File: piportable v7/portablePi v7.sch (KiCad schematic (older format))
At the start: 62 parts, among them IC1 Raspberry_Pi_Zero_W_(v1.3), J1 AudioJack3, SW0 SW_Push, SW1 SW_Push, SW10 SW_Push, SW11 SW_Push, SW12 SW_Push, SW13 SW_Push, SW14 SW_Push, SW15 SW_Push, SW16 SW_Push, SW17 SW_Push, SW18 SW_Push, SW19 SW_Push, SW2 SW_Push, SW20 SW_Push, SW21 SW_Push, SW22 SW_Push, SW23 SW_Push, SW24 SW_Push, SW25 SW_Push, SW26 SW_Push, SW27 SW_Push, SW28 SW_Push, SW29 SW_Push, SW3 SW_Push, SW30 SW_Push, SW31 SW_Push, SW32 SW_Push, SW33 SW_Push, SW34 SW_Push, SW35 SW_Push, SW36 SW_Push, SW37 SW_Push, SW38 SW_Push, SW39 SW_Push, SW4 SW_Push, SW40 SW_Push, SW41 SW_Push, SW42 SW_Push, SW43 SW_Push, SW44 SW_Push, SW45 SW_Push, SW46 SW_Push, SW47 SW_Push, SW48 SW_Push, SW49 SW_Push, SW5 SW_Push, SW50 SW_Push, SW51 SW_Push, SW52 SW_Push, SW53 SW_Push, SW54 SW_Push, SW55 SW_Push, SW56 SW_Push, SW6 SW_Push, SW7 SW_Push, SW8 SW_Push, SW9 SW_Push, U1 ATmega328P-PU

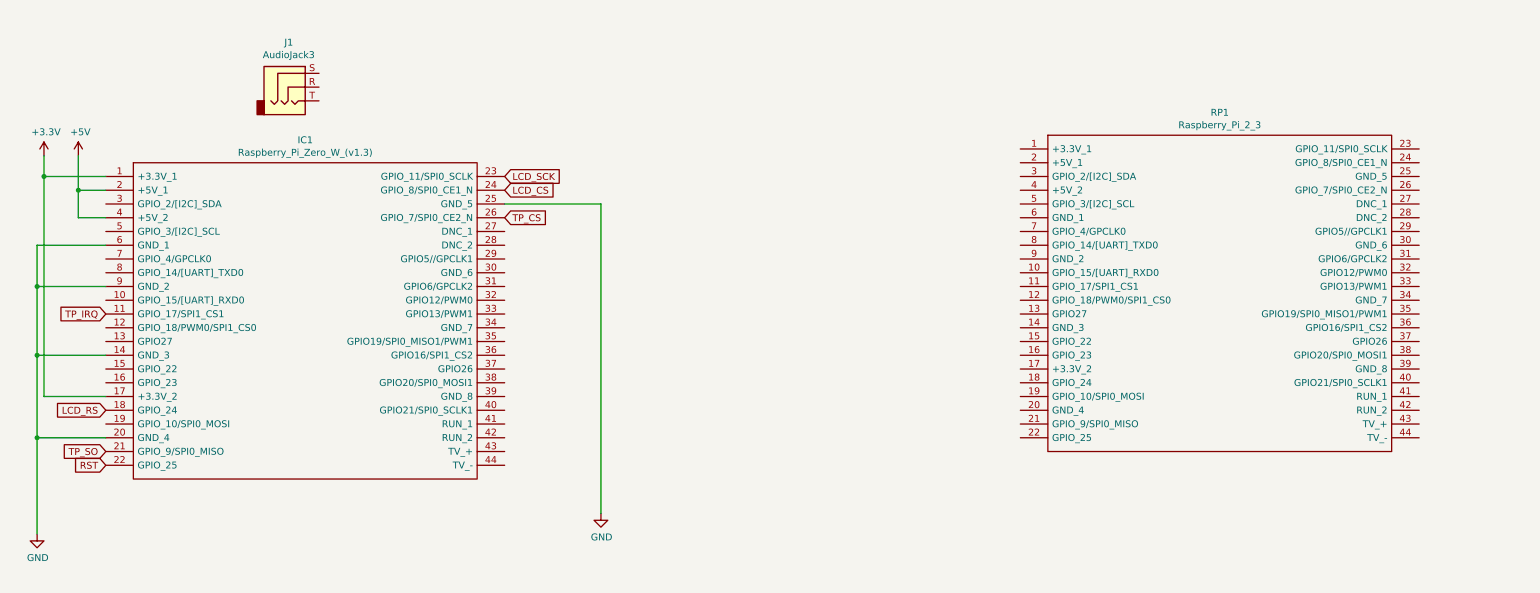
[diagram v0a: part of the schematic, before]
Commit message: nothing new
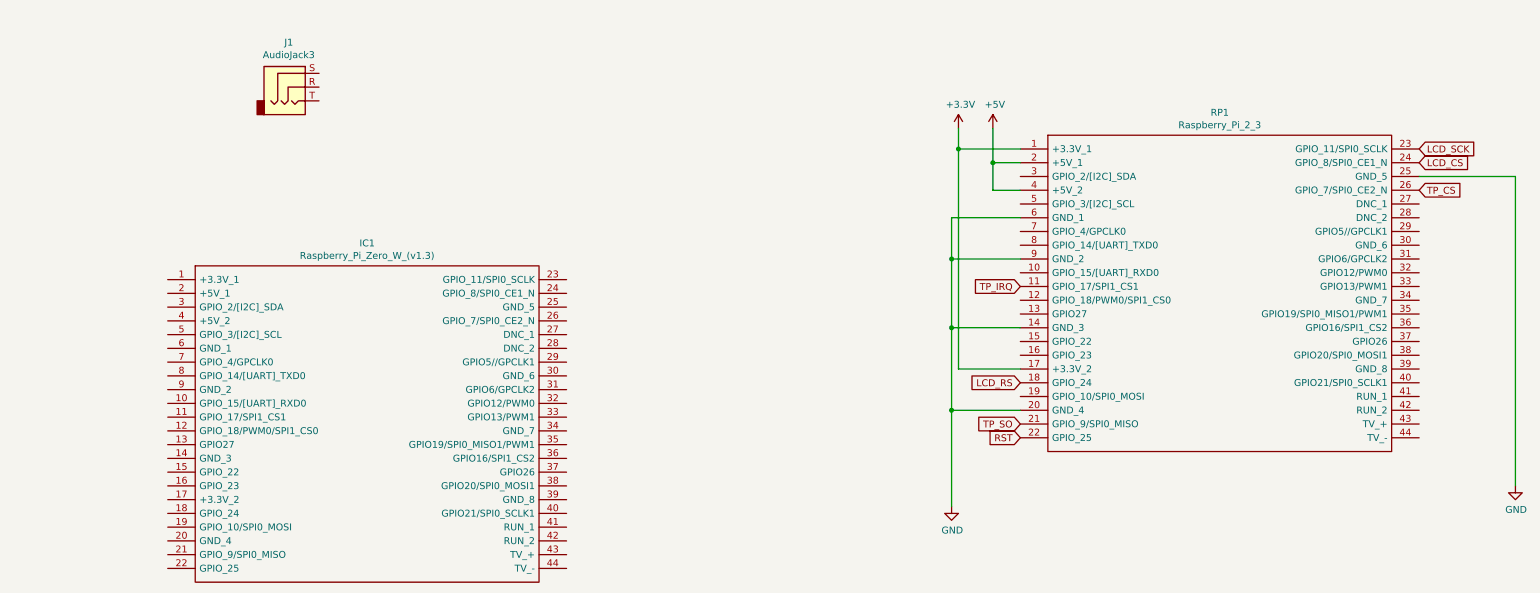
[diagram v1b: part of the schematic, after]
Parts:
- DS1: footprint pi2:raspberrypi_2_3 -> 35 display:3.5 inch RPi LCD
- RP1: footprint RASPBERRYPI -> (none)
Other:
- moved on the sheet: IC1
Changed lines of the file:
@@
 F 0 "DS1" H 2550 6647 50  0000 C CNN
 F 1 "3.5_Inch_RPI" H 2550 6556 50  0000 C CNN
-F 2 "pi2:raspberrypi_2_3" H 2550 5300 50  0001 C CNN
+F 2 "35 display:3.5 inch RPi LCD" H 2550 5300 50  0001 C CNN
 F 3 "DOCUMENTATION" H 2550 5300 50  0001 C CNN
 F 4 "https://www.elecrow.com/35-inch-480x320-tft-display-with-touch-screen-for-raspberry-pi-p-1385.html" H 2550 6465 50  0000 C CNN "Link"
@@
 L Raspberry_Pi_Zero_W_(v1.3):Raspberry_Pi_Zero_W_(v1.3) IC1
 U 1 1 5C56055C
-P 1350 7650
-F 0 "IC1" H 2800 7915 50  0000 C CNN
-F 1 "Raspberry_Pi_Zero_W_(v1.3)" H 2800 7824 50  0000 C CNN
-F 2 "pi2:raspberrypi_2_3" H 4100 7750 50  0001 L CNN
-F 3 "https://cdn.sparkfun.com/assets/learn_tutorials/6/7/6/PiZero_1.pdf" H 4100 7650 50  0001 L CNN
-F 4 "Raspberry Pi Zero W (v1.3) Single-board Computers" H 4100 7550 50  0001 L CNN "Description"
-F 5 "" H 4100 7450 50  0001 L CNN "Height"
-F 6 "RASPBERRY-PI" H 4100 7350 50  0001 L CNN "Manufacturer_Name"
-F 7 "Raspberry Pi Zero W (v1.3)" H 4100 7250 50  0001 L CNN "Manufacturer_Part_Number"
-F 8 "" H 4100 7150 50  0001 L CNN "RS Part Number"
-F 9 "" H 4100 7050 50  0001 L CNN "RS Price/Stock"
-F 10 "" H 4100 6950 50  0001 L CNN "Mouser Part Number"
-F 11 "" H 4100 6850 50  0001 L CNN "Mouser Price/Stock"
-	1    1350 7650
+P 1800 8400
+F 0 "IC1" H 3250 8665 50  0000 C CNN
+F 1 "Raspberry_Pi_Zero_W_(v1.3)" H 3250 8574 50  0000 C CNN
+F 2 "pi2:raspberrypi_2_3" H 4550 8500 50  0001 L CNN
+F 3 "https://cdn.sparkfun.com/assets/learn_tutorials/6/7/6/PiZero_1.pdf" H 4550 8400 50  0001 L CNN
+F 4 "Raspberry Pi Zero W (v1.3) Single-board Computers" H 4550 8300 50  0001 L CNN "Description"
+F 5 "" H 4550 8200 50  0001 L CNN "Height"
+F 6 "RASPBERRY-PI" H 4550 8100 50  0001 L CNN "Manufacturer_Name"
+F 7 "Raspberry Pi Zero W (v1.3)" H 4550 8000 50  0001 L CNN "Manufacturer_Part_Number"
+F 8 "" H 4550 7900 50  0001 L CNN "RS Part Number"
+F 9 "" H 4550 7800 50  0001 L CNN "RS Price/Stock"
+F 10 "" H 4550 7700 50  0001 L CNN "Mouser Part Number"
+F 11 "" H 4550 7600 50  0001 L CNN "Mouser Price/Stock"
+	1    1800 8400
 	1    0    0    -1
 $EndComp
@@
 Wire Wire Line
 	750  5800 750  6150
-Text GLabel 1350 9350 0    50   Input ~ 0
-LCD_RS
-Text GLabel 1350 9750 0    50   Input ~ 0
-RST
-Text GLabel 4250 7750 2    50   Input ~ 0
-LCD_CS
-Text GLabel 4250 7950 2    50   Input ~ 0
-TP_CS
-Text GLabel 1350 9650 0    50   Input ~ 0
-TP_SO
-Text GLabel 4250 7650 2    50   Input ~ 0
-LCD_SCK
-Text GLabel 1350 8650 0    50   Input ~ 0
-TP_IRQ
-$Comp
-L power:GND #PWR0105
-U 1 1 5C63ADD4
-P 4950 10100
-F 0 "#PWR0105" H 4950 9850 50  0001 C CNN
-F 1 "GND" H 4955 9927 50  0000 C CNN
-F 2 "" H 4950 10100 50  0001 C CNN
-F 3 "" H 4950 10100 50  0001 C CNN
-	1    4950 10100
-	1    0    0    -1
-$EndComp
-Wire Wire Line
-	4250 7850 4950 7850
-Wire Wire Line
-	4950 7850 4950 10100
-$Comp
-L power:GND #PWR0106
-U 1 1 5C641F49
-P 850 10250
-F 0 "#PWR0106" H 850 10000 50  0001 C CNN
-F 1 "GND" H 855 10077 50  0000 C CNN
-F 2 "" H 850 10250 50  0001 C CNN
-F 3 "" H 850 10250 50  0001 C CNN
-	1    850  10250
-	1    0    0    -1
-$EndComp
-Wire Wire Line
-	1350 9550 850  9550
-Wire Wire Line
-	850  9550 850  10250
-Wire Wire Line
-	1350 8950 850  8950
-Wire Wire Line
-	850  8950 850  9550
-Connection ~ 850  9550
-Wire Wire Line
-	1350 8450 850  8450
-Wire Wire Line
-	850  8450 850  8950
-Connection ~ 850  8950
-Wire Wire Line
-	1350 8150 850  8150
-Wire Wire Line
-	850  8150 850  8450
-Connection ~ 850  8450
-$Comp
-L power:+5V #PWR0107
-U 1 1 5C66060B
-P 1150 7500
-F 0 "#PWR0107" H 1150 7350 50  0001 C CNN
-F 1 "+5V" H 1165 7673 50  0000 C CNN
-F 2 "" H 1150 7500 50  0001 C CNN
-F 3 "" H 1150 7500 50  0001 C CNN
-	1    1150 7500
-	1    0    0    -1
-$EndComp
-Wire Wire Line
-	1150 7500 1150 7750
-Wire Wire Line
-	1150 7750 1350 7750
-Wire Wire Line
-	1350 7950 1150 7950
-Wire Wire Line
-	1150 7950 1150 7750
-Connection ~ 1150 7750
-$Comp
-L power:+3.3V #PWR0108
-U 1 1 5C678ACA
-P 900 7500
-F 0 "#PWR0108" H 900 7350 50  0001 C CNN
-F 1 "+3.3V" H 915 7673 50  0000 C CNN
-F 2 "" H 900 7500 50  0001 C CNN
-F 3 "" H 900 7500 50  0001 C CNN
-	1    900  7500
-	1    0    0    -1
-$EndComp
-Wire Wire Line
-	1350 7650 900  7650
-Wire Wire Line
-	900  7650 900  7500
-Wire Wire Line
-	1350 9250 900  9250
-Wire Wire Line
-	900  9250 900  7650
-Connection ~ 900  7650
 $Comp
 L portablePi-v7-rescue:Raspberry_Pi_2_3-Raspberry_Pi_2_or_3-portablePi-v5-rescue RP1
@@
 F 0 "RP1" H 9450 7715 50  0000 C CNN
 F 1 "Raspberry_Pi_2_3" H 9450 7624 50  0000 C CNN
-F 2 "RASPBERRYPI" H 9200 8350 50  0001 L CNN
+F 2 "" H 9200 8350 50  0001 L CNN
 F 3 "by lukaneco" H 9200 8050 50  0001 L CNN
 F 4 "Raspberry Pi Zero 2 or 3 Single-board Computers" H 9200 7950 50  0001 L CNN "Description"
@@
 	1    0    0    -1
 $EndComp
+Text GLabel 8000 9150 0    50   Input ~ 0
+LCD_RS
+Text GLabel 8000 9550 0    50   Input ~ 0
+RST
+Text GLabel 8000 9450 0    50   Input ~ 0
+TP_SO
+Text GLabel 8000 8450 0    50   Input ~ 0
+TP_IRQ
+$Comp
+L power:GND #PWR0105
+U 1 1 5C617599
+P 7500 10050
+F 0 "#PWR0105" H 7500 9800 50  0001 C CNN
+F 1 "GND" H 7505 9877 50  0000 C CNN
+F 2 "" H 7500 10050 50  0001 C CNN
+F 3 "" H 7500 10050 50  0001 C CNN
+	1    7500 10050
+	1    0    0    -1
+$EndComp
+Wire Wire Line
+	8000 9350 7500 9350
+Wire Wire Line
+	7500 9350 7500 10050
+Wire Wire Line
+	8000 8750 7500 8750
+Wire Wire Line
+	7500 8750 7500 9350
+Connection ~ 7500 9350
+Wire Wire Line
+	8000 8250 7500 8250
+Wire Wire Line
+	7500 8250 7500 8750
+Connection ~ 7500 8750
+Wire Wire Line
+	8000 7950 7500 7950
+Wire Wire Line
+	7500 7950 7500 8250
+Connection ~ 7500 8250
+$Comp
+L power:+5V #PWR0106
+U 1 1 5C6175AA
+P 7800 7300
+F 0 "#PWR0106" H 7800 7150 50  0001 C CNN
+F 1 "+5V" H 7815 7473 50  0000 C CNN
+F 2 "" H 7800 7300 50  0001 C CNN
+F 3 "" H 7800 7300 50  0001 C CNN
+	1    7800 7300
+	1    0    0    -1
+$EndComp
+Wire Wire Line
+	7800 7300 7800 7550
+Wire Wire Line
+	7800 7550 8000 7550
+Wire Wire Line
+	8000 7750 7800 7750
+Wire Wire Line
+	7800 7750 7800 7550
+Connection ~ 7800 7550
+$Comp
+L power:+3.3V #PWR0107
+U 1 1 5C6175B5
+P 7550 7300
+F 0 "#PWR0107" H 7550 7150 50  0001 C CNN
+F 1 "+3.3V" H 7565 7473 50  0000 C CNN
+F 2 "" H 7550 7300 50  0001 C CNN
+F 3 "" H 7550 7300 50  0001 C CNN
+	1    7550 7300
+	1    0    0    -1
+$EndComp
+Wire Wire Line
+	8000 7450 7550 7450
+Wire Wire Line
+	7550 7450 7550 7300
+Wire Wire Line
+	8000 9050 7550 9050
+Wire Wire Line
+	7550 9050 7550 7450
+Connection ~ 7550 7450
+Text GLabel 10900 7550 2    50   Input ~ 0
+LCD_CS
+Text GLabel 10900 7750 2    50   Input ~ 0
+TP_CS
+Text GLabel 10900 7450 2    50   Input ~ 0
+LCD_SCK
+$Comp
+L power:GND #PWR0108
+U 1 1 5C62C015
+P 11600 9900
+F 0 "#PWR0108" H 11600 9650 50  0001 C CNN
+F 1 "GND" H 11605 9727 50  0000 C CNN
+F 2 "" H 11600 9900 50  0001 C CNN
+F 3 "" H 11600 9900 50  0001 C CNN
+	1    11600 9900
+	1    0    0    -1
+$EndComp
+Wire Wire Line
+	10900 7650 11600 7650
+Wire Wire Line
+	11600 7650 11600 9900
 $EndSCHEMATC
